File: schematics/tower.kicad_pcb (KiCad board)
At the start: 2 copper layers, 50.8 x 48.3 mm, 17 parts, among them IC1 ESP32-SOLO-1, J1 Conn_01x02, J2 Conn_01x06, J3 Conn_01x09, J4 Conn_02x10_Odd_Even, SW1 SW_Push, SW2 SW_SPDT, U1 NCP1117-3.3_SOT223

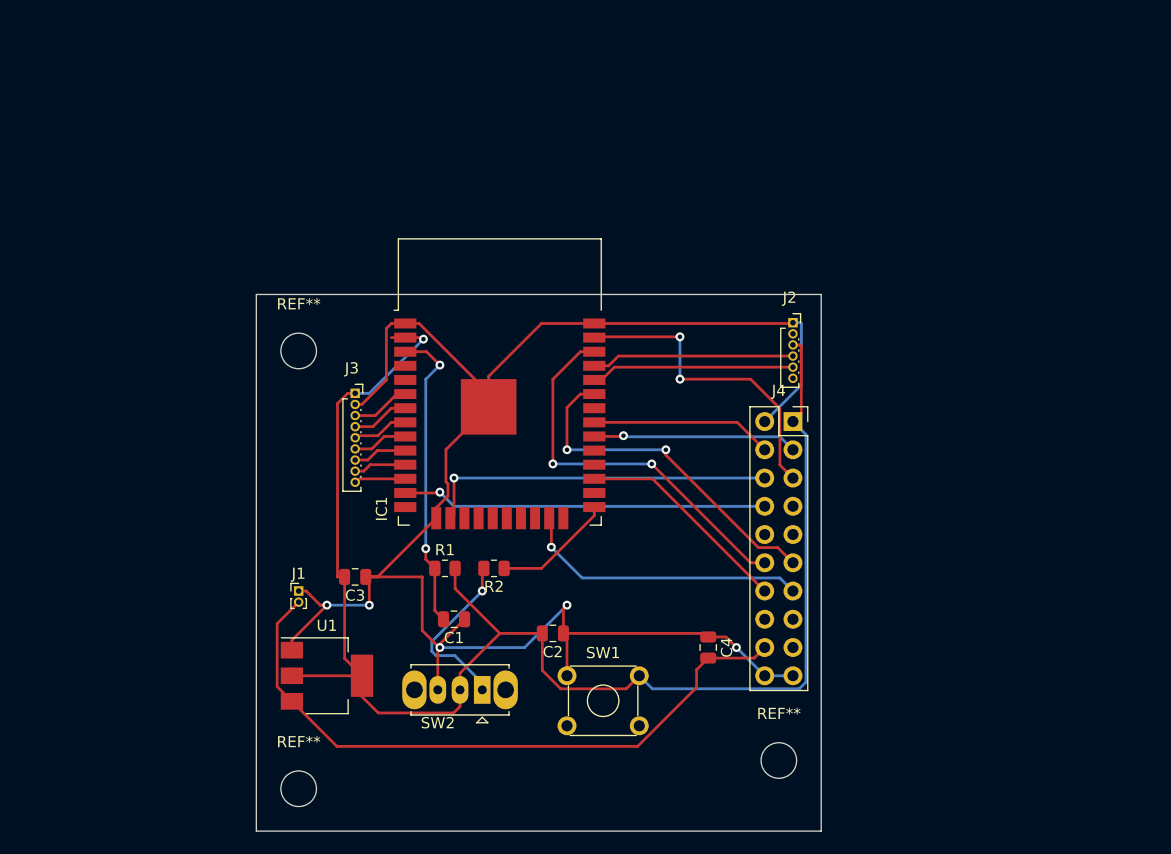
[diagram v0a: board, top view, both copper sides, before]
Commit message: finished (I think) schematics for tower and controller
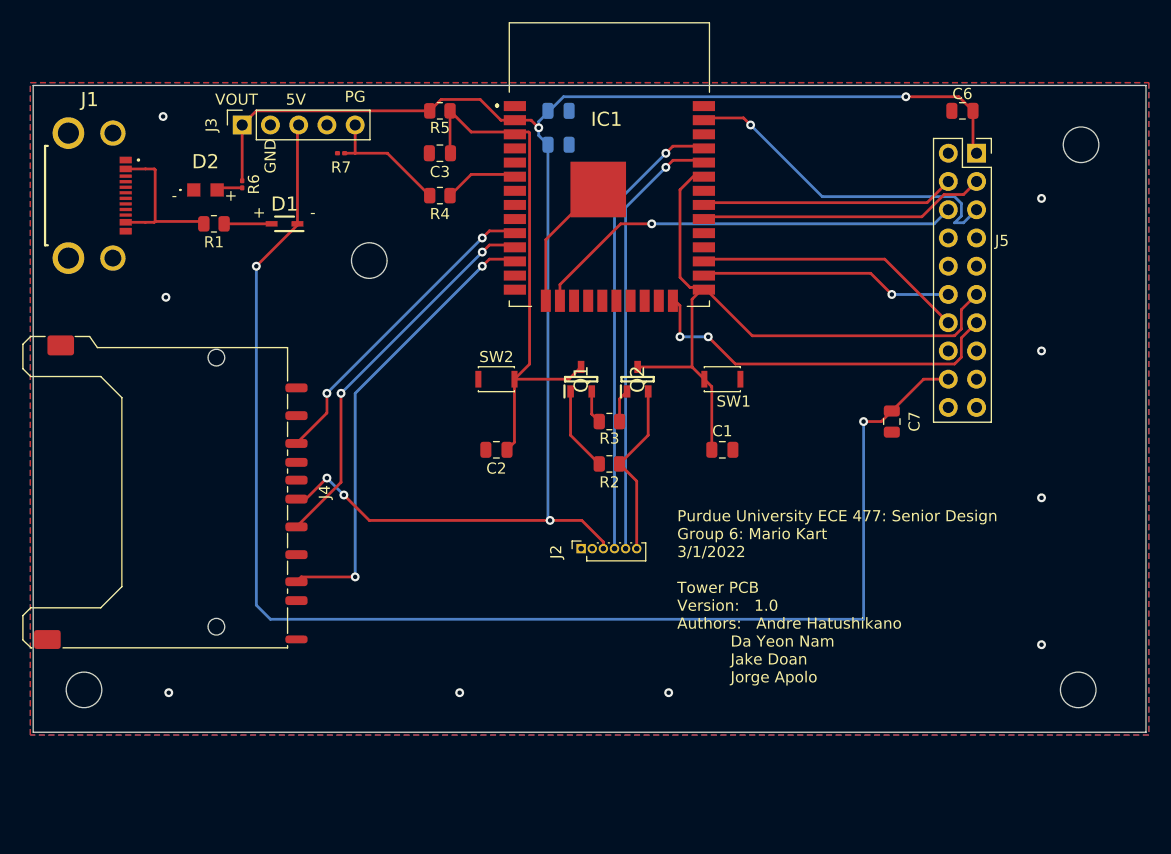
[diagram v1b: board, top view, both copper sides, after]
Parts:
- removed the REF** at (127.0, 119.4)
- removed the REF** at (170.2, 116.8)
- removed the REF** at (127.0, 80.0)
- removed U1: NCP1117-3.3_SOT223, Package_TO_SOT_SMD:SOT-223-3_TabPin2
- added C5: 100nF, Capacitor_SMD:C_0805_2012Metric, B.Cu at (150.4, 61.5)
- added C6: 100nF, Capacitor_SMD:C_0805_2012Metric, F.Cu at (186.7, 58.4)
- added C7: 100nF, Capacitor_SMD:C_0805_2012Metric, F.Cu at (180.3, 86.4)
- added D1: BAT760-7, Mouser:SOD2513X120N, F.Cu at (125.7, 68.6)
- added D2: LED, Mouser:APHCM2012QBCDF01, F.Cu at (118.6, 65.5)
- added J5: Conn_02x10_Odd_Even, Connector_PinSocket_2.54mm:PinSocket_2x10_P2.54mm_Vertical, F.Cu at (188.0, 62.2)
- added Q1: SS8050-G, Mouser:SOT95P240X115-3N, F.Cu at (152.4, 82.5)
- added Q2: SS8050-G, Mouser:SOT95P240X115-3N, F.Cu at (157.5, 82.5)
- added R3: 10k, Resistor_SMD:R_0805_2012Metric, F.Cu at (154.9, 86.4)
- added R4: 10k, Resistor_SMD:R_0805_2012Metric, F.Cu at (139.7, 66.0)
- added R5: 10k, Resistor_SMD:R_0805_2012Metric, F.Cu at (139.7, 58.4)
- added R6: 0, Resistor_SMD:R_0201_0603Metric, F.Cu at (121.9, 65.0)
- added R7: 0, Resistor_SMD:R_0201_0603Metric, F.Cu at (130.8, 62.2)
- added REF**: MountingHole_3.2mm_M3, MountingHole:MountingHole_3.2mm_M3, F.Cu at (133.3, 71.9)
- added REF**: MountingHole_3.2mm_M3, MountingHole:MountingHole_3.2mm_M3, F.Cu at (197.4, 61.5)
- added REF**: MountingHole_3.2mm_M3, MountingHole:MountingHole_3.2mm_M3, F.Cu at (197.1, 110.5)
- added REF**: MountingHole_3.2mm_M3, MountingHole:MountingHole_3.2mm_M3, F.Cu at (107.7, 110.5)
- C1, C2: value 100nF -> 0.1uF
- C4: value 100nF -> 22uF; moved to B.Cu
- IC1: footprint RF_Module:ESP32-WROOM-32 -> Mouser:ESP32SOLO1
- J1: value Conn_01x02 -> 216990-0003; footprint Connector_PinHeader_1.00mm:PinHeader_1x02_P1.00mm_Vertical -> Mouser:2169900003
- J3: value Conn_01x09 -> Conn_01x05; footprint Connector_PinSocket_1.00mm:PinSocket_1x09_P1.00mm_Vertical -> Connector_PinSocket_2.54mm:PinSocket_1x05_P2.54mm_Vertical
- J4: value Conn_02x10_Odd_Even -> SD_Card; footprint Connector_PinSocket_2.54mm:PinSocket_2x10_P2.54mm_Vertical -> Connector_Card:SD_Kyocera_145638109211859+
- R1: value 10k -> 20
- SW1: footprint Button_Switch_THT:SW_TH_Tactile_Omron_B3F-10xx -> Button_Switch_SMD:SW_SPST_CK_KXT3
- SW2: value SW_SPDT -> SW_Push; footprint Button_Switch_THT:SW_Slide_1P2T_CK_OS102011MS2Q -> Button_Switch_SMD:SW_SPST_CK_KXT3
- moved J4 57.5 mm to (114.3, 92.7), turned to 270 degrees
- moved C4 50.1 mm to (150.4, 58.4), turned to 0 degrees
- moved J1 40.6 mm to (107.4, 66.0), turned to 270 degrees
- moved C3 38.9 mm to (139.7, 62.2)
- moved R1 37.3 mm to (119.4, 68.6), turned to 180 degrees
- moved SW1 30.1 mm to (165.1, 82.5), turned to 180 degrees
- moved C1 28.5 mm to (165.1, 88.9), turned to 0 degrees
- moved SW2 28.0 mm to (144.8, 82.5), turned to 0 degrees
- moved J2 27.9 mm to (152.4, 97.8), turned to 90 degrees
- moved J3 26.2 mm to (121.9, 59.7), turned to 90 degrees
- moved IC1 24.4 mm to (154.9, 63.5)
- moved C2 17.3 mm to (144.8, 88.9)
- moved R2 14.0 mm to (154.9, 90.2)
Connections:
- net AUDIO_L renamed Net-(J4-Pad9)
- C1 pad 1: GND -> GPIO0
- C1 pad 2: Net-(C1-Pad2) -> GND
- C2 pad 1: GND -> EN
- C2 pad 2: Vcc -> GND
- C3 pad 1: GND -> EN
- C3 pad 2: Vcc -> GND
- C4 pad 1: GND -> VOUT
- C4 pad 2: 5V -> GND
- IC1 pad 10: IO25 -> SDMOSI
- IC1 pad 11: IO26 -> SDCLK
- IC1 pad 12: IO27 -> SDMISO
- IC1 pad 13: PDN -> Net-(IC1-Pad13)
- IC1 pad 2: Vcc -> VOUT
- IC1 pad 23: GPIO2 -> Net-(IC1-Pad23)
- IC1 pad 24: Net-(IC1-Pad24) -> GPIO2
- IC1 pad 25: Net-(IC1-Pad25) -> GPIO0
- IC1 pad 26: Net-(IC1-Pad26) -> GPIO1
- IC1 pad 28: DTR -> Net-(IC1-Pad28)
- IC1 pad 29: CTS -> Net-(IC1-Pad29)
- IC1 pad 3: Net-(C1-Pad2) -> EN
- IC1 pad 36: GPIO1 -> Net-(IC1-Pad36)
- J2 pad 3: Vcc -> VOUT
- J3 pad 1: Vcc -> VOUT
- J3 pad 3: IO34 -> 5V
- J3 pad 4: IO35 -> SHDN
- J3 pad 5: IO32 -> PG
- J4 pad 1: Vcc -> Net-(J4-Pad1)
- J4 pad 10: NC -> Net-(J4-Pad10)
- J4 pad 11: GPIO0 -> Net-(J4-Pad11)
- J4 pad 12: GPIO1 -> Net-(J4-Pad12)
- J4 pad 13: GPIO2 -> Net-(J4-Pad13)
- J4 pad 2: GND -> SDMOSI
- J4 pad 3: SCK -> GND
- J4 pad 4: MISO -> VOUT
- J4 pad 5: MOSI -> SDCLK
- J4 pad 6: CS -> GND
- J4 pad 7: INT -> SDMISO
- J4 pad 8: PDN -> Net-(J4-Pad8)
- R1 pad 1: Net-(C1-Pad2) -> Net-(D1-Pad2)
- R1 pad 2: Vcc -> Net-(J1-PadA4)
- R2 pad 1: Net-(IC1-Pad25) -> DTR
- R2 pad 2: Net-(R2-Pad2) -> Net-(Q1-Pad1)
- SW1 pad 2: Vcc -> GPIO0
- SW2 pad 1: Net-(R2-Pad2) -> GND
- SW2 pad 2: Vcc -> EN
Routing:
- net GND: track 161.6 -> 14.6 mm, vias 5 -> 9
- net VOUT: track 0.00 -> 146.3 mm, vias 0 -> 5
- net Vcc: track 136.8 -> 0.00 mm, vias 1 -> 0
- net 5V: track 59.5 -> 126.9 mm, vias 0 -> 2
- net EN: track 0.00 -> 47.6 mm
- net SDMISO: track 0.00 -> 41.3 mm, vias 0 -> 2
- net SDCLK: track 0.00 -> 34.8 mm, vias 0 -> 2
- net PDN: track 32.9 -> 0.00 mm, vias 1 -> 0
- net GPIO0: track 31.6 -> 62.7 mm, vias 2 -> 0
- net SDMOSI: track 0.00 -> 28.6 mm, vias 0 -> 2
- net Net-(C1-Pad2): track 27.7 -> 0.00 mm, vias 2 -> 0
- net TX: track 18.2 -> 41.2 mm, vias 0 -> 1
- net RX: track 18.3 -> 39.5 mm, vias 0 -> 1
- net DTR: track 0.00 -> 15.8 mm
- net Net-(R2-Pad2): track 15.7 -> 0.00 mm, vias 1 -> 0
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- added copper zone on B.Cu, net GND
- added copper zone on F.Cu, net GND
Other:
- board size 50.8 x 48.3 mm -> 100.1 x 58.2 mm
- board text added: "+"
- board text added: "-"
- board text added: "5V"
- board text added: "GND"
- board text added: "PG"
- board text added: "Purdue University ECE 477: Senior Design Group 6: Mario Kart 3/1/2022 Tower PCB Version: 1.0 Authors: Andre Hatushikano Da Yeon Nam Jake Doan Jorge Apolo"
- board text added: "VOUT"
